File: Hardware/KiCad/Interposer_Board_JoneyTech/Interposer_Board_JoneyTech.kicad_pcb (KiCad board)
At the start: 4 copper layers, 122.5 x 99.5 mm, 6 parts, among them J1 M.2 Key M, J2 M.2 Key M

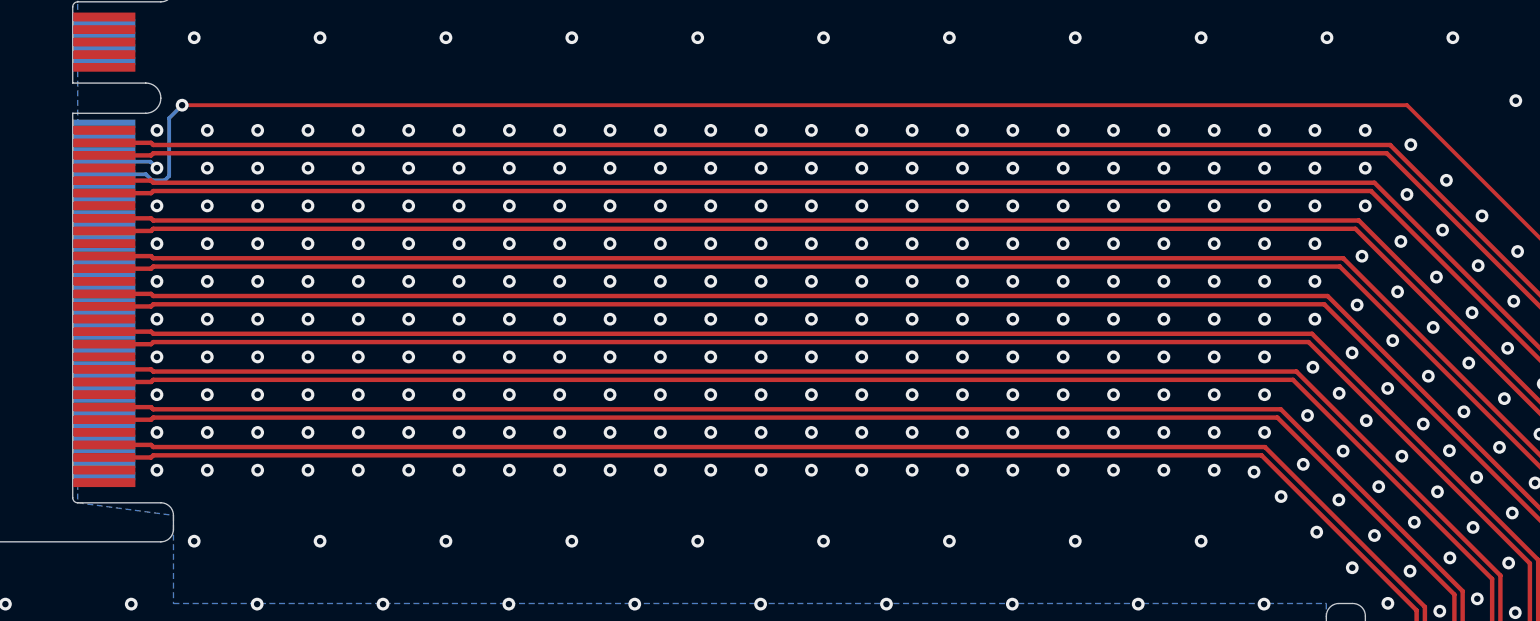
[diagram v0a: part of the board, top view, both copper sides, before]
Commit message: JoneyTech Interposer Diff Pairs Skew Matched
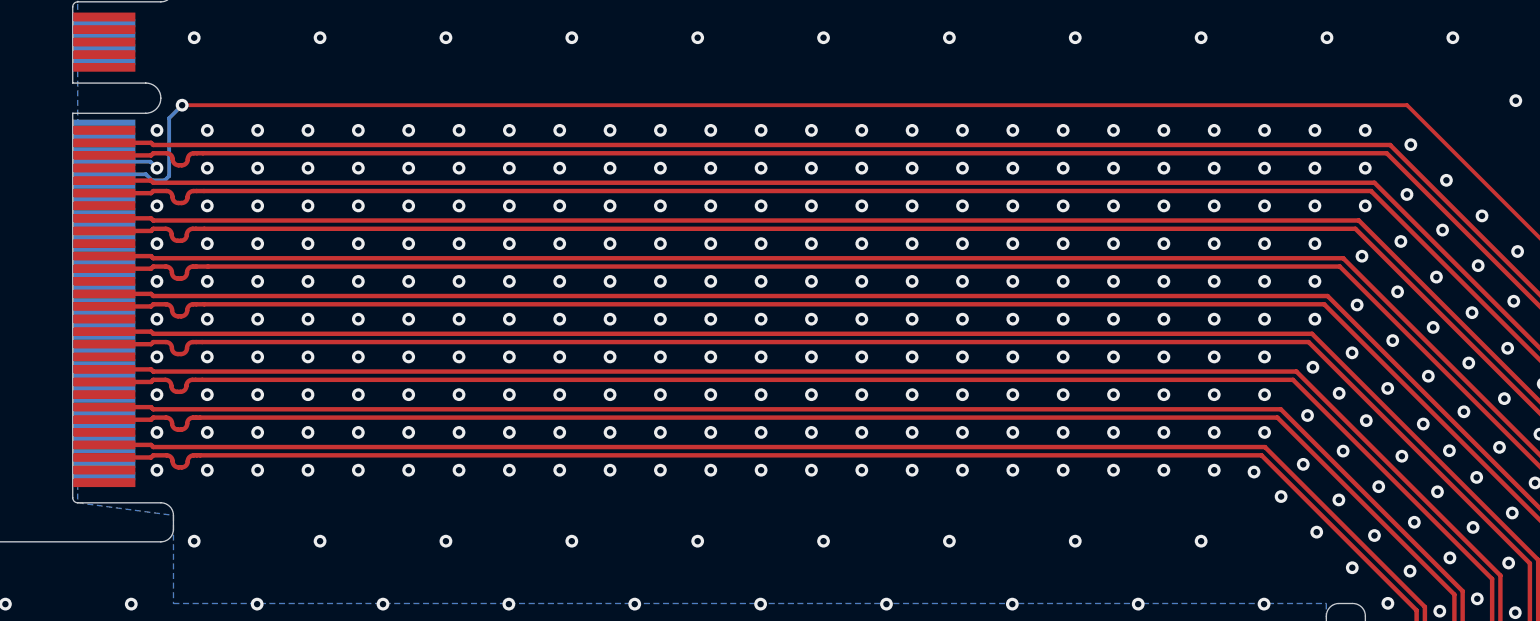
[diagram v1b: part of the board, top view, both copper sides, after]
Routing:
- net /RX3_N: track 59.7 -> 60.2 mm
- net /RX0_N: track 74.6 -> 75.1 mm
- net /TX3_N: track 57.2 -> 57.8 mm
- net /RX1_N: track 69.7 -> 70.2 mm
- net /REFCLK_N: track 77.1 -> 77.6 mm
- net /TX1_N: track 67.2 -> 67.7 mm
- net /RX2_N: track 64.7 -> 65.2 mm
- net /TX2_N: track 62.2 -> 62.7 mm
- net /TX0_N: track 72.2 -> 72.7 mm

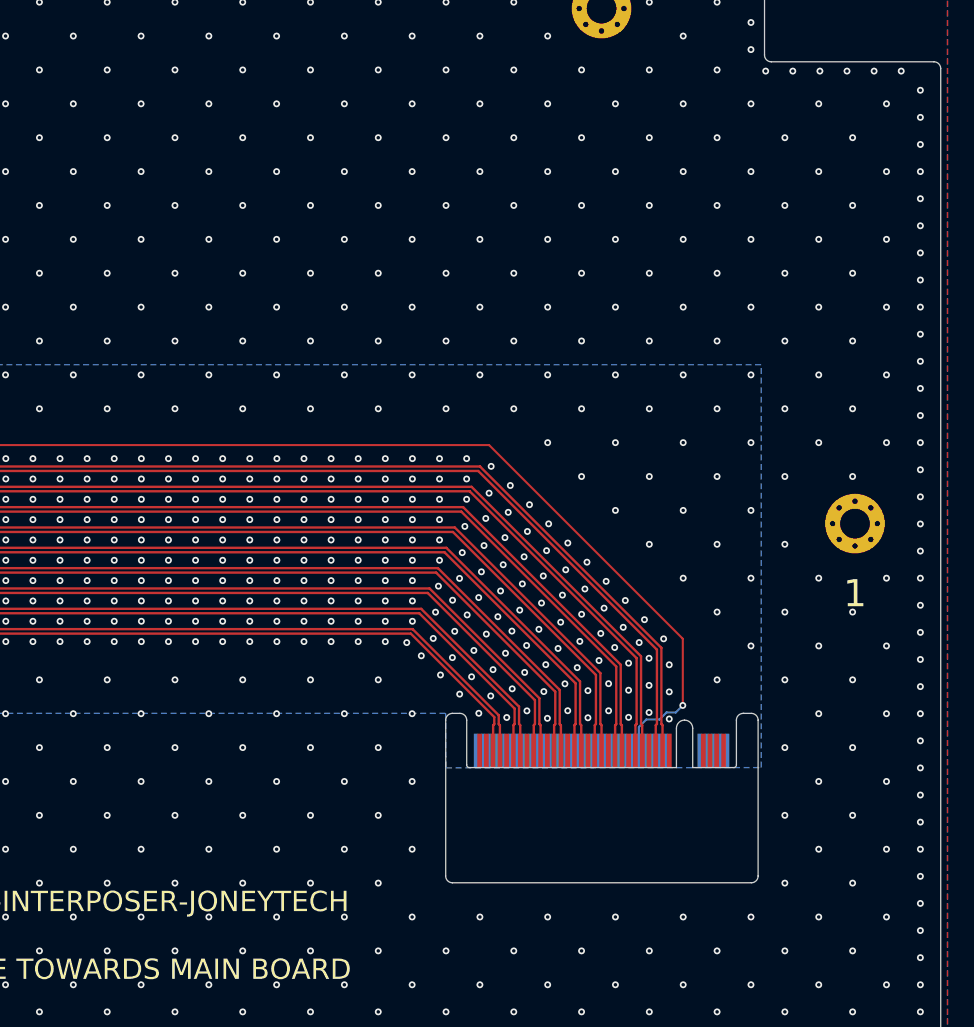
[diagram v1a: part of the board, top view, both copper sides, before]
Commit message: Fixed Hole Spacing on IOCrest Interposer
Also added clearance holes for heatsink push pins and grounding lug
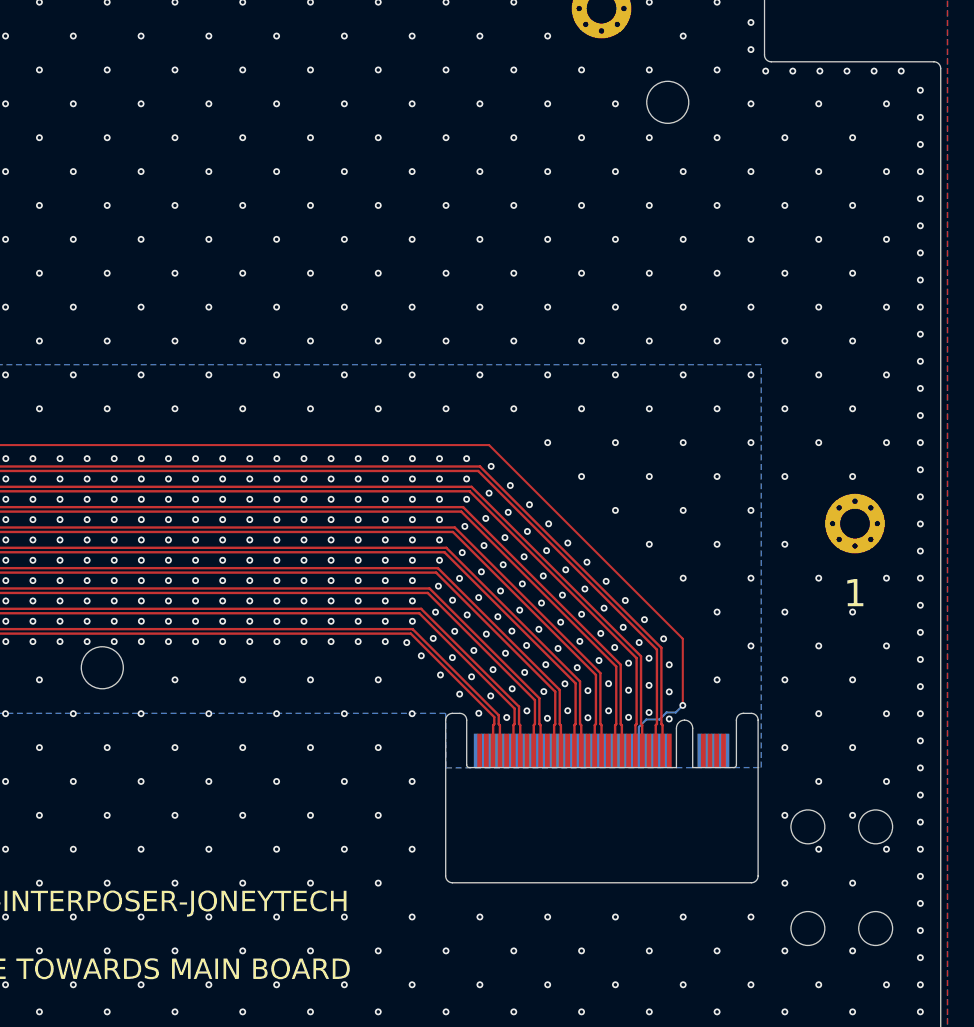
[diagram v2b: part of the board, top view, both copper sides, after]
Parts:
- added HS1: HSB30-373710, ThunderScope:SSKY_HSB30-373710_MountingHoles, F.Cu at (151.3, 70.1)
- added J11: 7793, ThunderScope:KEY_7792_ClearenceHoles, F.Cu at (185.0, 106.5)
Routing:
- net GND: vias 1191 -> 1187
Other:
- board text added: "Differential trace width is 0.17644 mm and spacing is 0.127mm target impedance is 85 Ohm differential and tolerance is 10% traces are on top copper and reference is on inner layer 1"
